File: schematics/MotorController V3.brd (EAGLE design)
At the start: 120.6 x 100 mm, 54 parts, among them IC1 7805, Q1 BC307

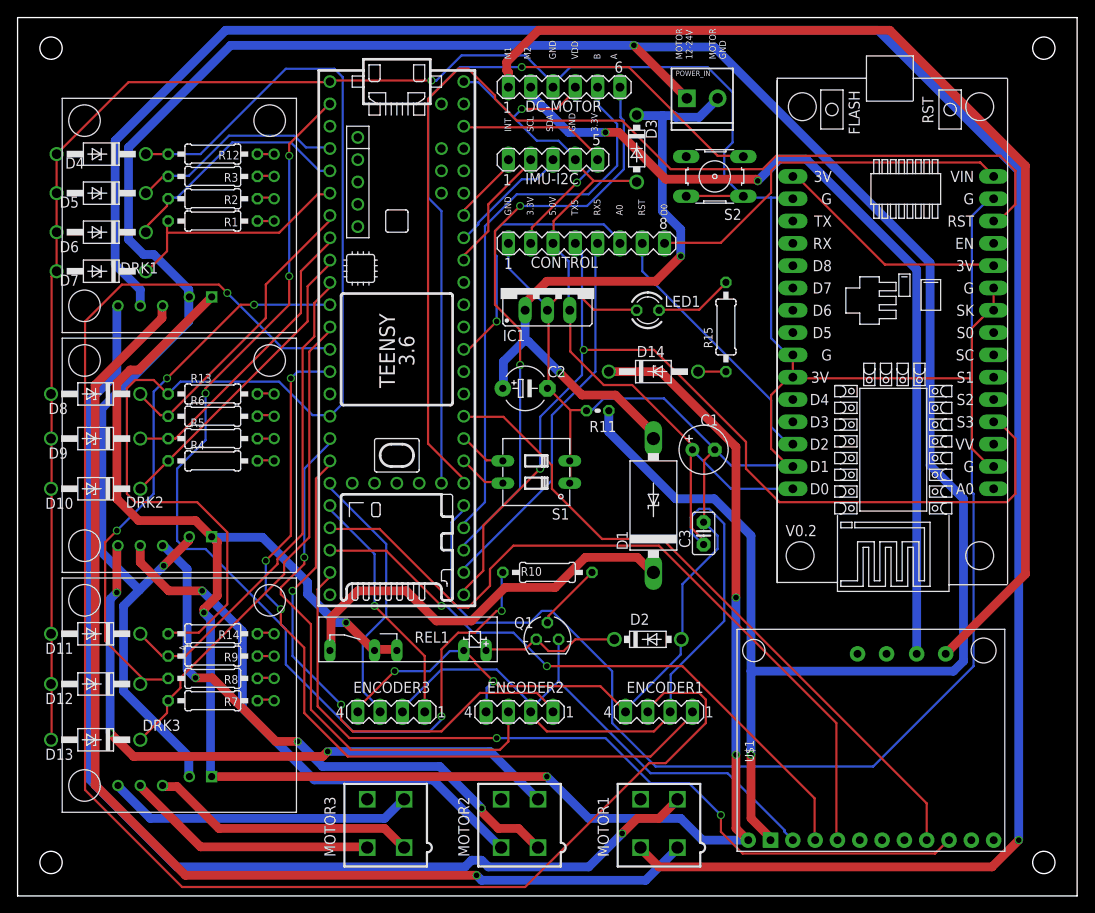
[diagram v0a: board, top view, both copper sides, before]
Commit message: no message
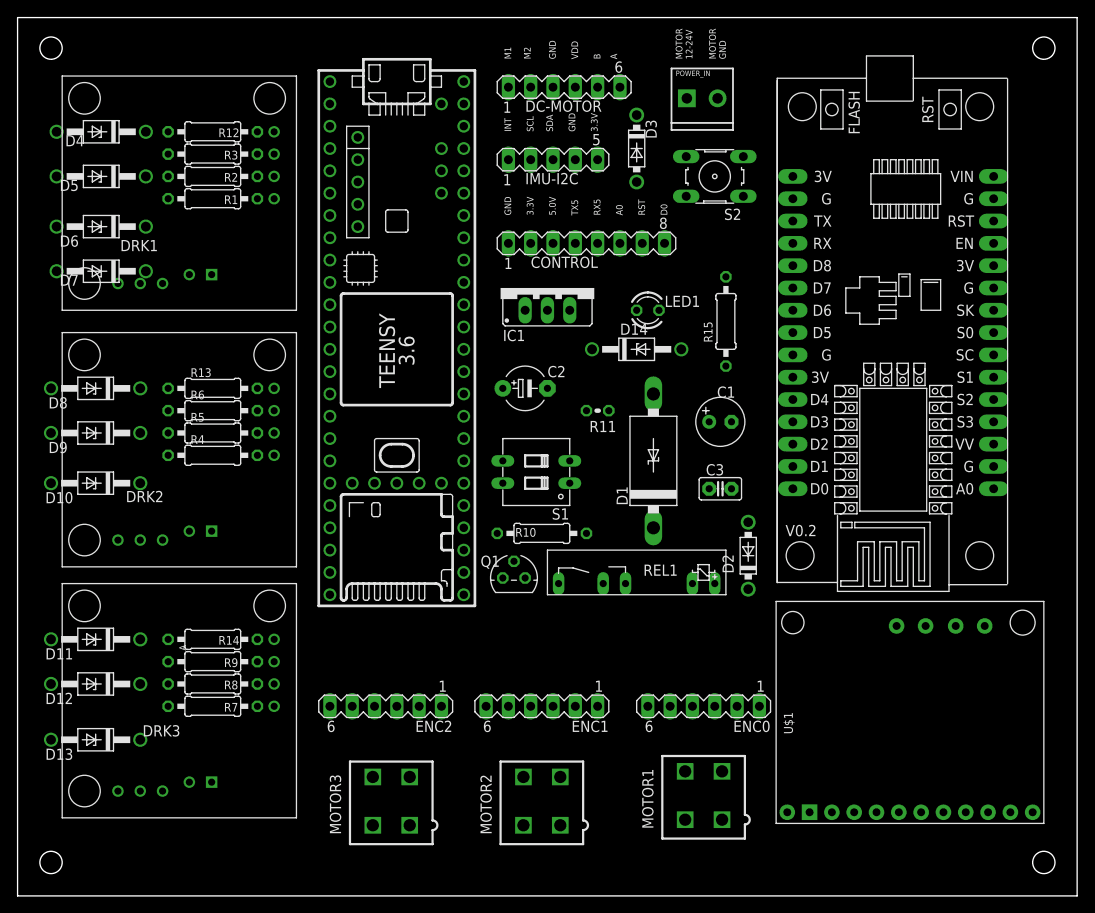
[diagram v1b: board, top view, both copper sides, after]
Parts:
- removed ENCODER1, ENCODER2, ENCODER3: 1, con-lstb:MA04-1
- added ENC0, ENC1, ENC2: (no value), con-lstb:MA06-1
- moved REL1 27.1 mm to (-3.17, 21.6)
- moved D2 14.9 mm to (8.26, 24.8), turned to 90 degrees
- moved Q1 7.96 mm to (-18.4, 22.2)
- moved MOTOR1 5.99 mm to (3.17, -2.54)
- moved U$1 5.46 mm to (25.4, -0.64)
- moved C3 5.43 mm to (5.08, 32.4), turned to 0 degrees
- moved D1 5.08 mm to (-2.54, 35.6)
- moved R10 4.49 mm to (-15.2, 27.3)
- moved C1 3.70 mm to (5.08, 40.0)
- moved MOTOR2 3.59 mm to (-15.2, -3.17)
- moved D14 3.17 mm to (-4.45, 48.3)
- moved MOTOR3 2.62 mm to (-32.4, -3.17)
- moved D4 2.54 mm to (-65.4, 73.0)
- moved R12 2.54 mm to (-52.7, 73.0)
- moved R3 2.54 mm to (-52.7, 70.5)
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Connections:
- removed net +5V: C1.+, C3.1, CONTROL.3, D3.A, DC-MOTOR.4, ENCODER1.2, ENCODER2.2, ENCODER3.2, IC1.OUT, IMU-I2C.4, PRJ1.VIN, Q1.1, U$1.VDD(5V), U$2.30
- removed net ENC1_A: ENCODER1.3, PRJ1.11/MOSI
- removed net ENC1_B: ENCODER1.1, PRJ1.12/MISO
- removed net ENC2_A: ENCODER2.3, PRJ1.25
- removed net ENC2_B: ENCODER2.1, PRJ1.26
- removed net ENC3_A: ENCODER3.3, PRJ1.27
- removed net ENC3_B: ENCODER3.1, PRJ1.28
- new net +3.6V: C1.+, C3.1, CONTROL.3, D3.A, DC-MOTOR.4, IC1.OUT, IMU-I2C.4, PRJ1.VIN, Q1.1, U$1.VDD(5V), U$2.30
- new net CS0: ENC0.2, PRJ1.26
- new net CS1: ENC1.2, PRJ1.25
- new net CS2: ENC2.2, PRJ1.28
- new net MISO: ENC0.5, ENC1.5, ENC2.5, PRJ1.12/MISO
- new net MOSI: ENC0.4, ENC1.4, ENC2.4, PRJ1.11/MOSI
- new net SCK: ENC0.3, ENC1.3, ENC2.3, PRJ1.27
- net 3.3V: now also ENC0.1, ENC1.1, ENC2.1
- net GND: now also ENC0.6, ENC1.6, ENC2.6; no longer ENCODER1.4, ENCODER2.4, ENCODER3.4
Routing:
- net GND: track 404.5 -> 0.00 mm, vias 3 -> 0
- net LIPO-GND: track 338.9 -> 0.00 mm, vias 3 -> 0
- net N$2: track 256.2 -> 0.00 mm, vias 1 -> 0
- net LIPO-VDD: track 224.2 -> 0.00 mm, vias 5 -> 0
- net +5V: track 213.6 -> 0.00 mm, vias 1 -> 0
- net ENC1_A: track 179.7 -> 0.00 mm, vias 1 -> 0
- net SDA1: track 142.7 -> 0.00 mm
- net N$46: track 134.0 -> 0.00 mm
- net N$1: track 130.3 -> 0.00 mm, vias 1 -> 0
- net N$3: track 130.1 -> 0.00 mm, vias 1 -> 0
- net RED-M1: track 129.2 -> 0.00 mm
- net SCL1: track 127.1 -> 0.00 mm
- net N$42: track 120.1 -> 0.00 mm, vias 5 -> 0
- net TX5: track 114.2 -> 0.00 mm, vias 2 -> 0
- net BLCK-M2: track 98.9 -> 0.00 mm, vias 2 -> 0
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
